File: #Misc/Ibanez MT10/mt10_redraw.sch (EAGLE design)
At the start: 60 parts, among them Q1 2SK184-GR, Q2 2SK184-GR, Q3 2SK184-GR, Q4 2SK184-GR, Q5 2SK184-GR, Q6 2N3906-, Q7 2SK184-GR

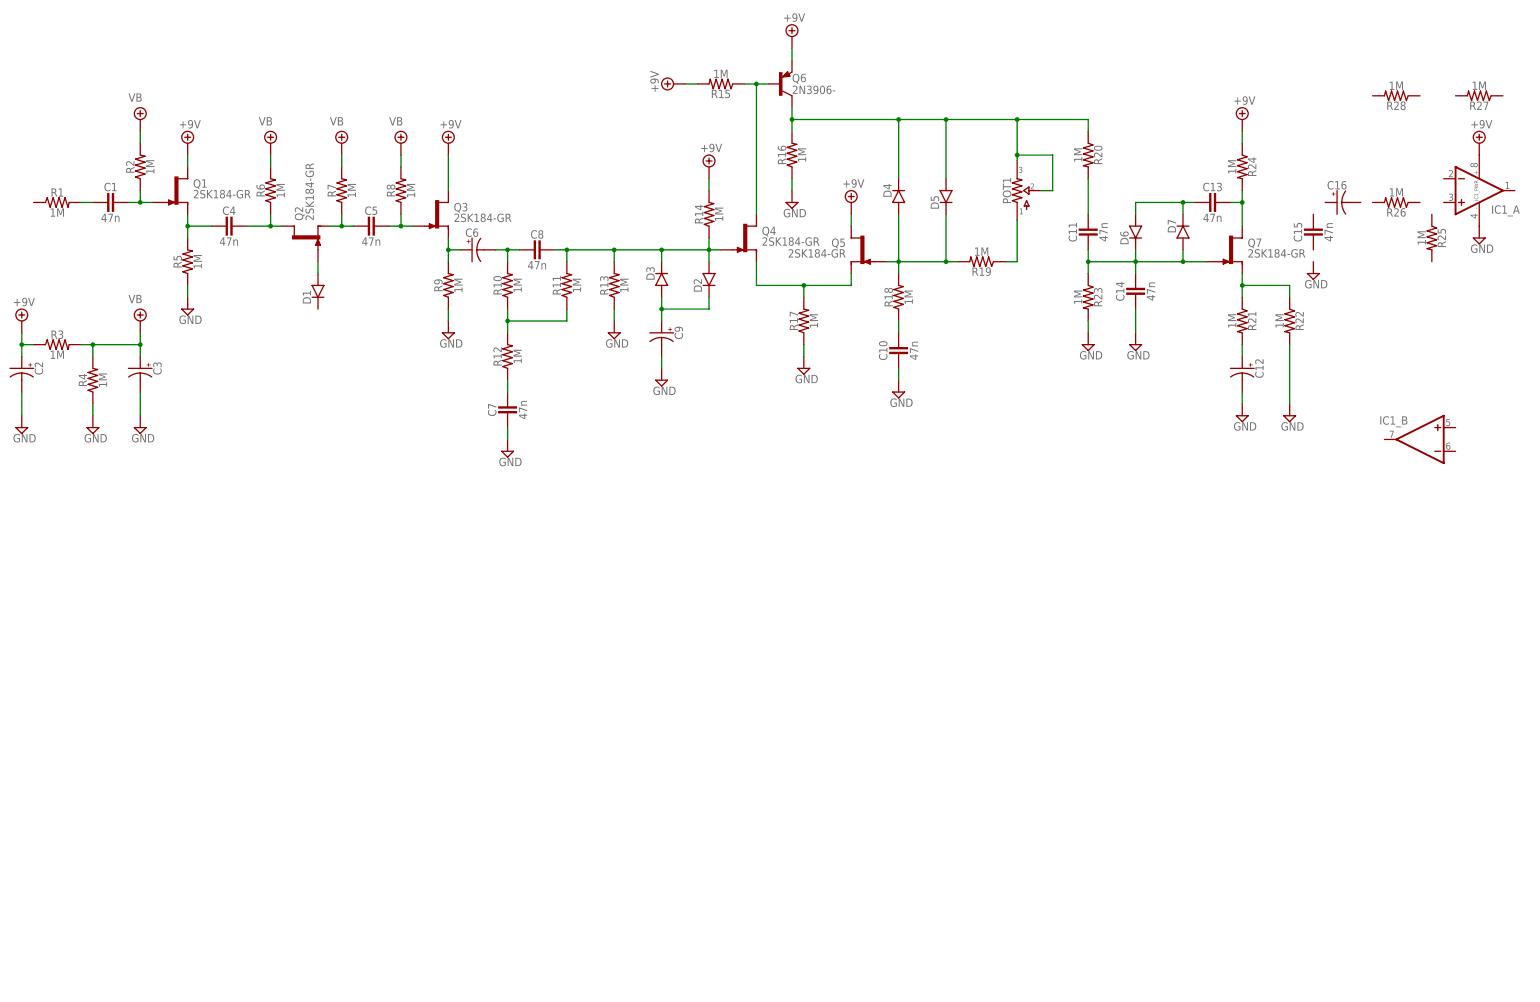
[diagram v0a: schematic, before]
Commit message: 20180102
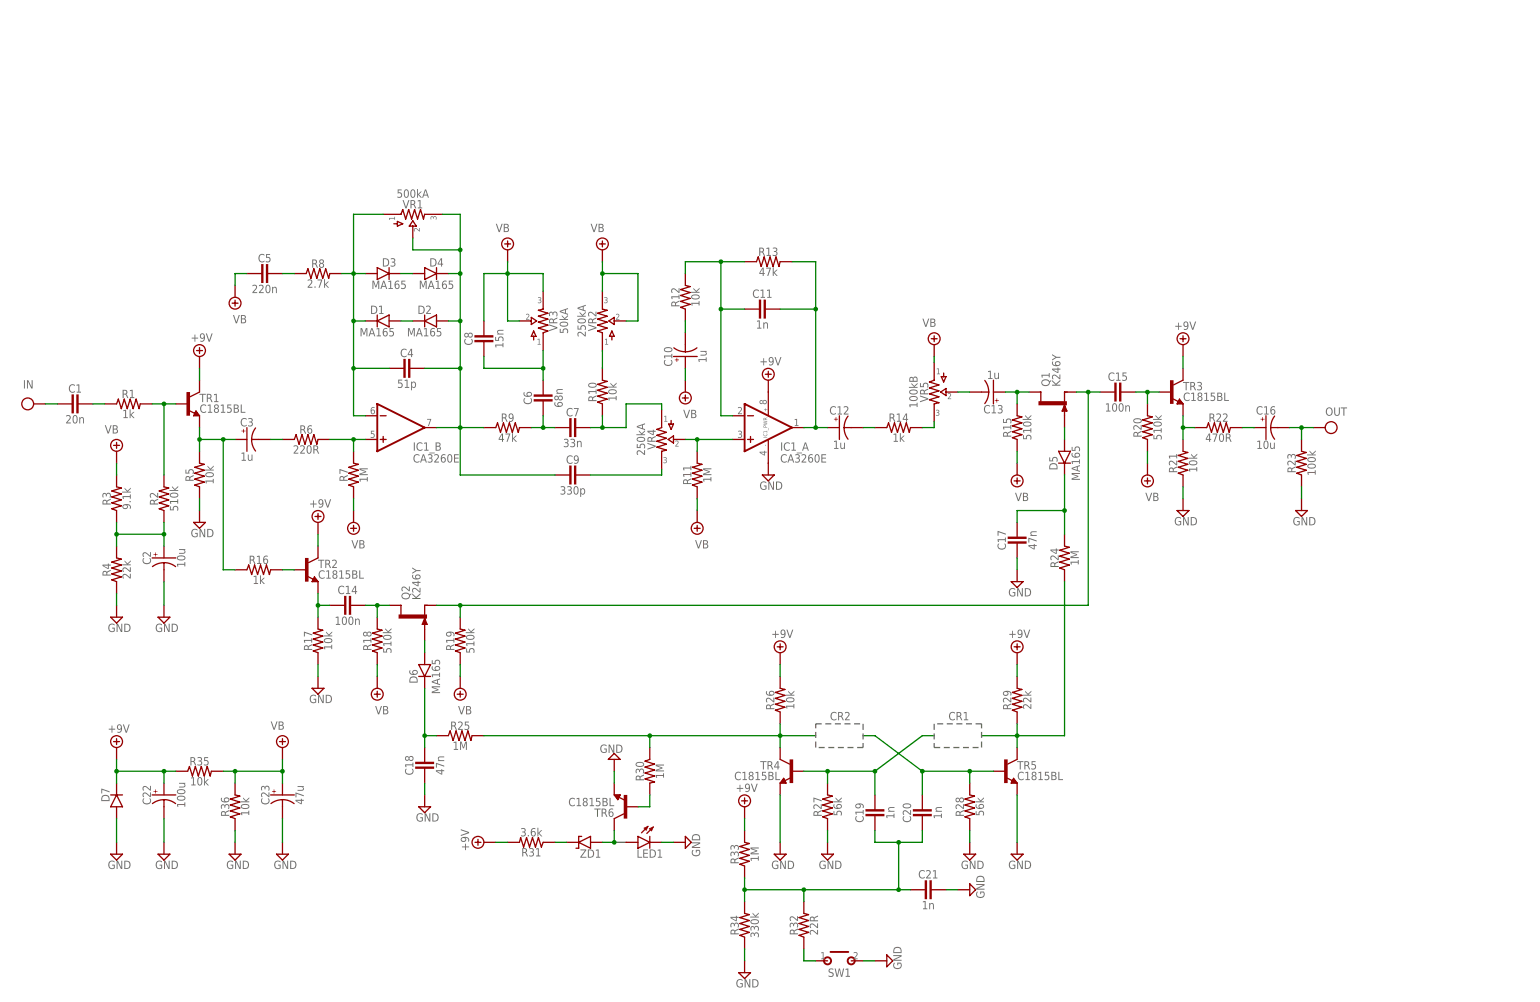
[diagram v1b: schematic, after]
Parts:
- removed POT1: (no value), pedals-potentiometers:POTS16MM
- removed Q3, Q4, Q5, Q7: 2SK184-GR, pedals-transistors:2N3819TO-92S
- removed Q6: 2N3906-, pedals-transistors:2N3906-
- added C17, C18: 47n, pedals-capacitors-film:CER/FILMBOX.1
- added C19, C20, C21: 1n, pedals-capacitors-film:CER/FILMBOX.1
- added C22: 100u, pedals-capacitors-elec:0500
- added C23: 47u, pedals-capacitors-elec:0500
- added LED1: LED, pedals-diodes:LED
- added R29: 22k, pedals-resistors:R_.3B
- added R30, R33: 1M, pedals-resistors:R_.3B
- added R31: 3.6k, pedals-resistors:R_.3B
- added R32: 22R, pedals-resistors:R_.3B
- added R34: 330k, pedals-resistors:R_.3B
- added R35, R36: 10k, pedals-resistors:R_.3B
- added SW1: MOMENTARY, pedals-switches:MOMENTARY
- added TR1, TR2, TR3, TR4, TR5, TR6: C1815BL, pedals-transistors:2SC828A
- added VR1: 500kA, pedals-potentiometers:POTS16MM
- added VR2, VR4: 250kA, pedals-potentiometers:POTS16MM
- added VR3: 50kA, pedals-potentiometers:POTS16MM
- added VR5: 100kB, pedals-potentiometers:POTS16MM
- added ZD1: (no value), pedals-diodes:ZENER.1
- C1: value 47n -> 20n
- C10, C13: value 47n -> 1u; device pedals-capacitors-film:CER/FILMBOX.1 -> pedals-capacitors-elec:0500
- C11: value 47n -> 1n
- C12, C3: value (none) -> 1u
- C14, C15: value 47n -> 100n
- C16, C2: value (none) -> 10u
- C4: value 47n -> 51p
- C5: value 47n -> 220n
- C6: value (none) -> 68n; device pedals-capacitors-elec:0500 -> pedals-capacitors-film:CER/FILMBOX.1
- C7: value 47n -> 33n
- C8: value 47n -> 15n
- C9: value (none) -> 330p; device pedals-capacitors-elec:0500 -> pedals-capacitors-film:CER/FILMBOX.1
- D1, D2, D3, D4, D5, D6: value (none) -> MA165
- IC1: value (none) -> CA3260E
- Q1, Q2: value 2SK184-GR -> K246Y; device pedals-transistors:2N3819TO-92S -> pedals-transistors:2N5457
- R1, R14, R16: value 1M -> 1k
- R10, R12, R17, R21, R26, R5: value 1M -> 10k
- R13, R9: value 1M -> 47k
- R15, R18, R19, R2, R20: value 1M -> 510k
- R22: value 1M -> 470R
- R23: value 1M -> 100k
- R27, R28: value 1M -> 56k
- R3: value 1M -> 9.1k
- R4: value 1M -> 22k
- R6: value 1M -> 220R
- R8: value 1M -> 2.7k
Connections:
- new net IN: C1.2
- new net N$20: C10.-, R12.1
- new net N$27: C15.2, Q1.S, Q2.S, R19.2
- new net N$28: C14.2, R17.2, TR2.E
- new net N$29: C19.2, C20.2, C21.1, R32.2, R33.1, R34.2
- new net N$30: C14.1, Q2.D, R18.2
- new net N$31: R24.1, R29.1, TR5.C
- new net N$32: C19.1, R27.2, TR4.B
- new net N$33: D6.A, Q2.G
- new net N$34: C20.1, R28.2, TR5.B
- new net N$35: C9.1, VR4.3
- new net N$38: TR6.C, ZD1.A
- new net N$39: R25.2, R26.1, R30.1, TR4.C
- new net N$40: R31.1, ZD1.C
- new net N$41: D5.A, Q1.G
- new net N$42: C17.1, D5.C, R24.2
- new net N$43: R32.1, SW1.P
- new net N$45: C16.+, R22.2
- new net N$46: R21.2, R22.1, TR3.E
- new net N$47: C15.1, R20.2, TR3.B
- new net OUT: C16.-, R23.2
- net +9V: now also C22.+, D7.C, R26.2, R29.2, R31.2, R33.2, R35.1, TR1.C, TR2.C, TR3.C; no longer C2.+, Q1.D, Q3.D, Q5.D, Q6.E, R14.2, R15.2, R24.1, R3.1
- net GND: now also C17.2, C18.2, C21.2, C22.-, C23.-, D7.A, LED1.C, R21.1, R23.1, R27.1, R28.1, R34.1, R36.1, SW1.S, TR4.E, TR5.E, TR6.E; no longer C10.2, C12.-, C14.2, C3.-, C7.2, C9.-, R13.1, R16.1, R22.2, R23.2, R9.1
- net N$1: now also C7.1, R10.1, VR4.1; no longer C9.+, D2.C, D3.A
- net N$10: now also IC1_B.+IN, R6.2, R7.2; no longer C6.+, Q3.S, R9.2
- net N$11: now also D1.A, D2.C; no longer C6.-, C8.2, R10.2
- net N$12: now also C5.1, R8.1; no longer R10.1, R11.1, R12.2
- net N$13: now also D4.A; no longer C8.1, D2.A, Q4.G, R11.2, R13.2, R14.1
- net N$14: now also R10.2, VR2.1; no longer C7.1, R12.1
- net N$15: now also TR2.B; no longer D4.C, D5.A, POT1.2, POT1.3, Q6.C, R20.1
- net N$16: now also C12.-, R14.1; no longer Q4.S, Q5.S, R17.2
- net N$17: now also R14.2, VR5.3; no longer D4.A, D5.C, Q5.G, R18.2, R19.2
- net N$18: now also C6.1, C8.2, VR3.1; no longer C10.1, R18.1
- net N$19: now also IC1_A.+IN, R11.2, VR4.2; no longer POT1.1, R19.1
- net N$2: now also C4.1, C9.2, D2.A, D4.C, IC1_B.OUT, R9.1, VR1.2, VR1.3; no longer Q4.D, Q6.B, R15.1
- net N$21: now also C11.2, IC1_A.-IN, R12.2, R13.1; no longer C11.1, R20.2
- net N$22: now also C11.1, C12.+, IC1_A.OUT, R13.2; no longer C11.2, C14.1, D6.C, D7.A, Q7.G, R23.1
- net N$23: now also C13.-, VR5.2; no longer C13.1, Q7.D, R24.2
- net N$24: now also R30.2, TR6.B; no longer C13.2, D6.A, D7.C
- net N$25: now also C13.+, Q1.D, R15.2; no longer C12.+, R21.2
- net N$26: now also C18.1, D6.C, R25.1; no longer Q7.S, R21.1, R22.1
- net N$3: now also C1.1, R1.1; no longer C1.2, R1.2
- net N$4: now also R1.2, R2.2, TR1.B; no longer C1.1, Q1.G, R2.1
- net N$5: now also C2.+, R2.1, R3.1, R4.2; no longer C4.2, Q1.S, R5.2
- net N$6: now also C3.+, R16.1, R5.2, TR1.E; no longer C4.1, Q2.D, R6.1
- net N$7: now also C4.2, D1.C, D3.A, IC1_B.-IN, R8.2, VR1.1; no longer C5.2, Q2.S, R7.1
- net N$8: now also C6.2, C7.2, R9.2; no longer C5.1, Q3.G, R8.1
- net N$9: now also C3.-, R6.1; no longer D1.A, Q2.G
- net VB: now also C10.+, C23.+, C5.2, C8.1, R11.1, R15.1, R18.1, R19.1, R20.1, R35.2, R36.2, R7.1, VR2.2, VR2.3, VR3.2, VR3.3, VR5.1; no longer C3.+, R2.2, R4.2, R6.2, R7.2, R8.2
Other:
- note added: "CR1"
- note added: "CR2"
- moved on the sheet: C1, C11, C12, C14, C15, C16, C2, C3, C4, C5, C7, C8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
